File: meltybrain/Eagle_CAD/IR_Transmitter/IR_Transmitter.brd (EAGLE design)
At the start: 33.2 x 27.6 mm, 14 parts, among them J1 AVR_SPI_PROG_3X2NS, Q1 BSS806N, Q2 FDN352AP, U1 LMH6612MAX/NOPB, U2 AP2210K-5.0TRG1

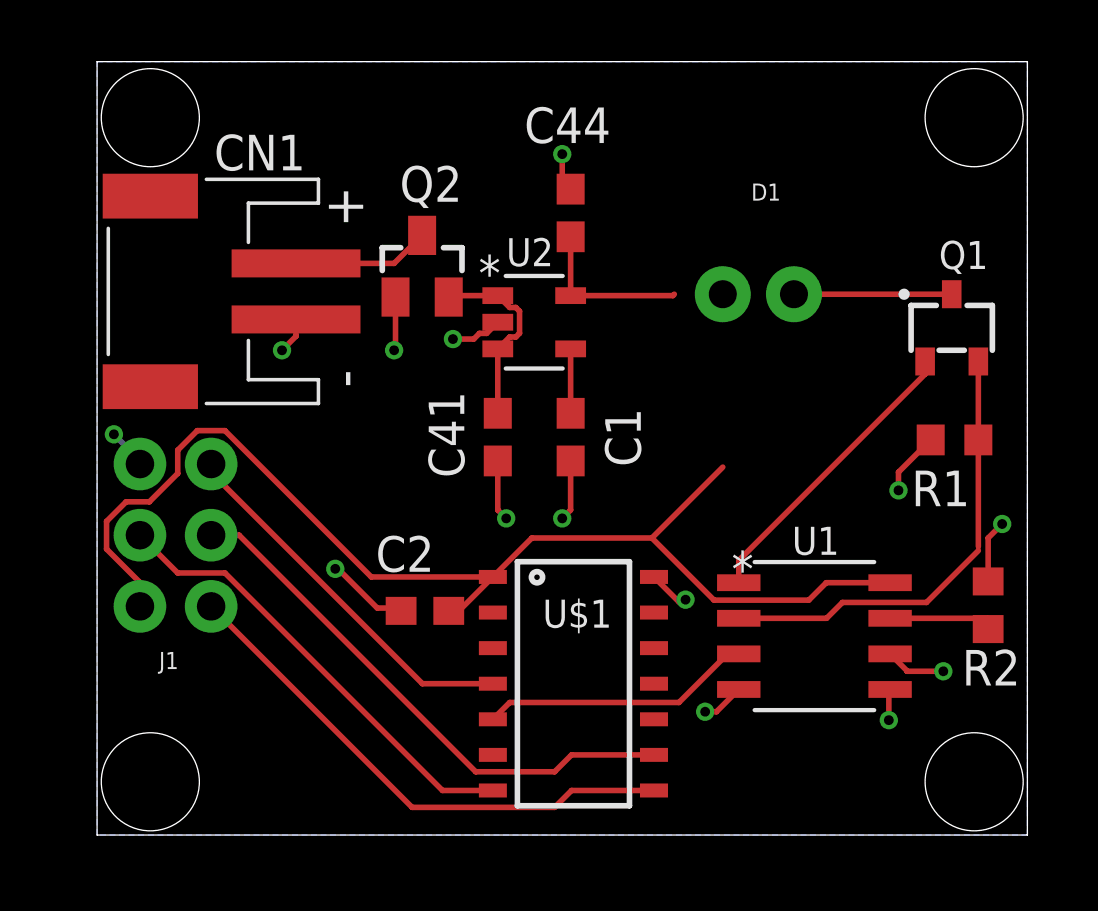
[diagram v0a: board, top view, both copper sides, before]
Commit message: Finalized emitter board
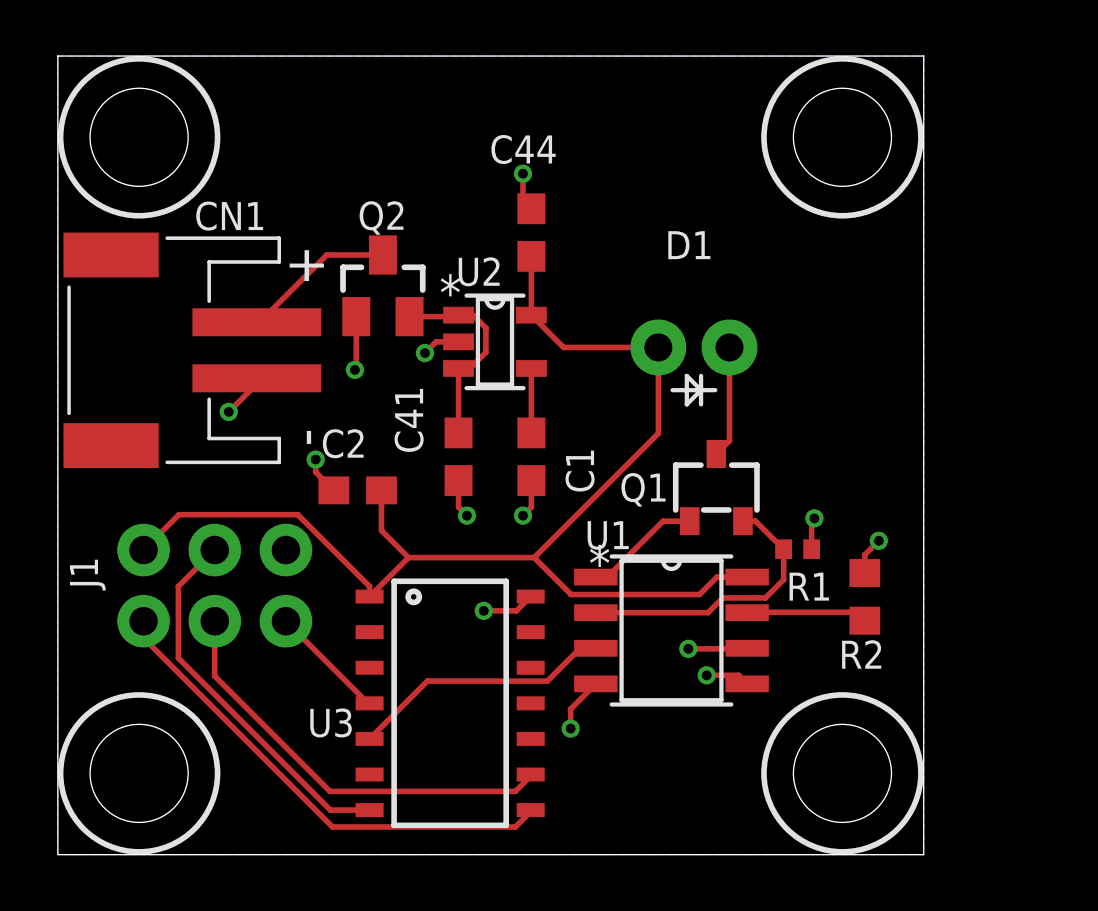
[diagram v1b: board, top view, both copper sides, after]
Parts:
- removed U$1: ATTINY84, EmitterParts:SOIC-14
- added U3: ATTINY84, EmitterParts:SOIC-14
- R1: value 6.8 -> 1.5; device rcl:R0603 -> rcl:R0402
- moved Q1 10.2 mm to (23.5, 13.1)
- moved R1 6.82 mm to (26.4, 10.9), turned to 180 degrees
- moved U1 5.10 mm to (21.9, 8.00)
- moved C2 4.92 mm to (10.7, 13.0)
- moved R2 4.41 mm to (28.8, 9.20)
- moved D1 2.98 mm to (22.7, 18.1)
- moved CN1 2.52 mm to (3.40, 18.0)
- moved J1 2.28 mm to (5.60, 9.60), turned to 0 degrees
- moved C1 1.57 mm to (16.9, 14.2)
- moved C44 1.57 mm to (16.9, 22.2)
- moved Q2 1.57 mm to (11.6, 20.3)
- moved U2 1.57 mm to (15.6, 18.3)
- moved C41 1.57 mm to (14.3, 14.2)
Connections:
- net +5V: now also U3.1; no longer U$1.1
- net GND: now also U3.14; no longer U$1.14
- net MISO: now also U3.8; no longer U$1.8
- net MOSI: now also U3.7; no longer U$1.7
- net OUT: now also U3.5; no longer U$1.5
- net RST: now also U3.4; no longer U$1.4
- net SCK: now also U3.9; no longer U$1.9
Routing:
- net RST: track 13.5 -> 4.20 mm
- net N$2: track 10.6 -> 4.18 mm
- net N$1: track 16.3 -> 10.1 mm
- net GND: track 26.2 -> 20.5 mm, vias 14 -> 13
- net +5V: track 48.7 -> 44.1 mm
- net SCK: track 19.6 -> 15.2 mm
- net MOSI: track 16.4 -> 13.5 mm
- net N$5: track 5.63 -> 3.99 mm
- net MISO: track 19.0 -> 17.5 mm
- net N$3: track 3.88 -> 4.48 mm
- net 9V: track 4.91 -> 5.49 mm
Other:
- board size 33.2 x 27.6 mm -> 30.9 x 28.5 mm
